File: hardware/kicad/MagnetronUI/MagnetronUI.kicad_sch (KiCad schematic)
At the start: 7 parts, among them J1 Conn_01x04, J2 Conn_02x13_Counter_Clockwise, SW1 SW_Push

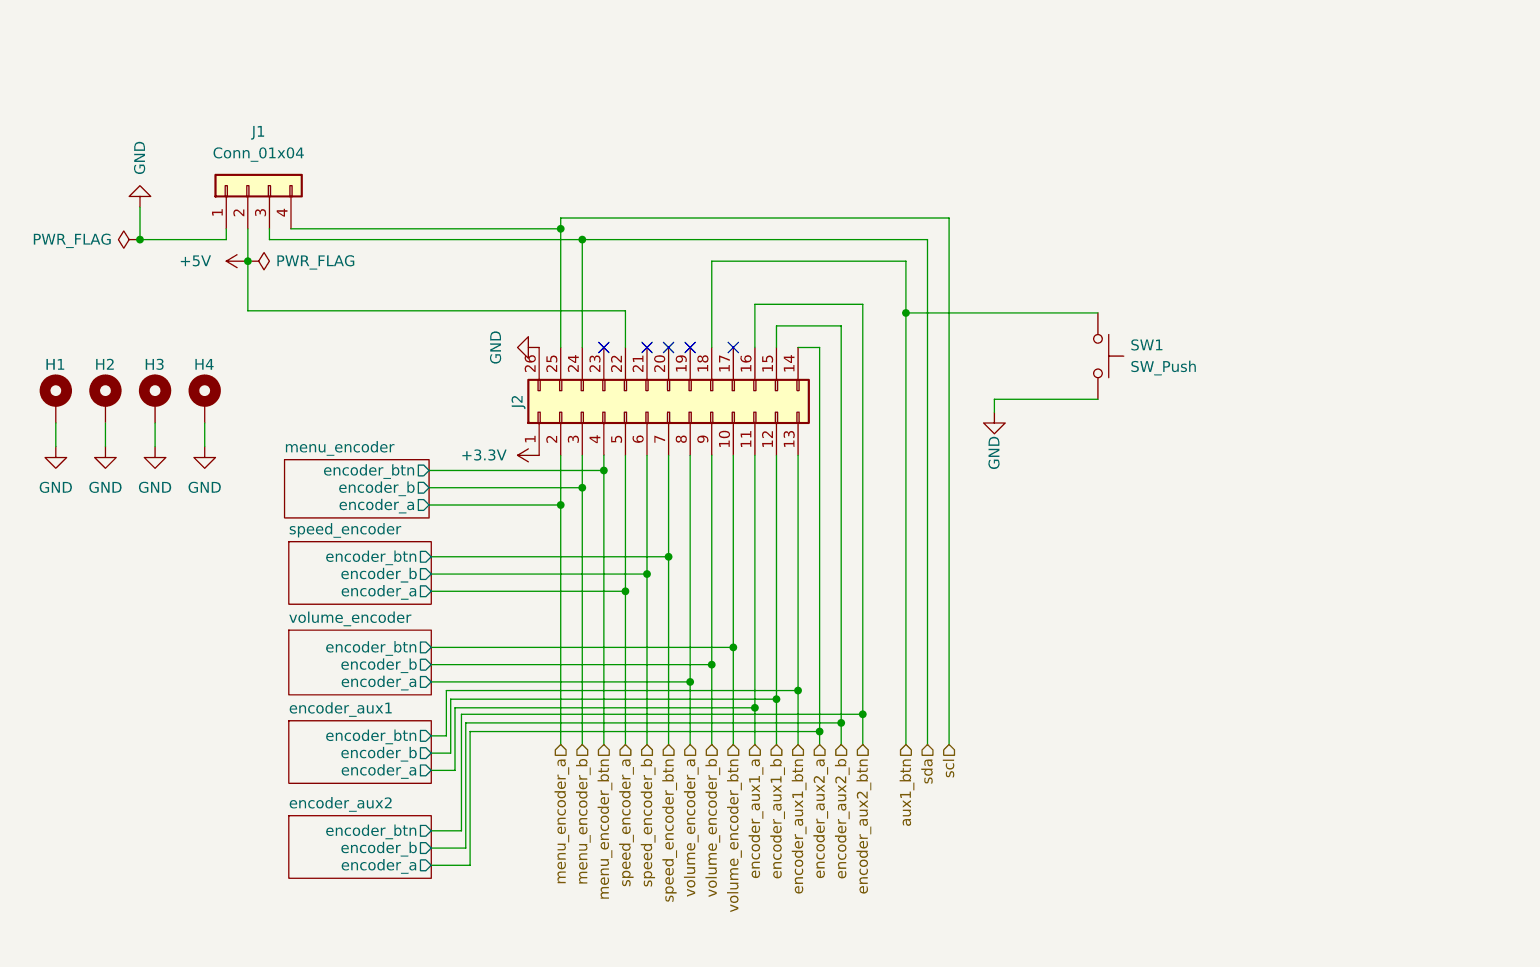
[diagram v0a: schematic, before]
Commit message: chore: cleanup
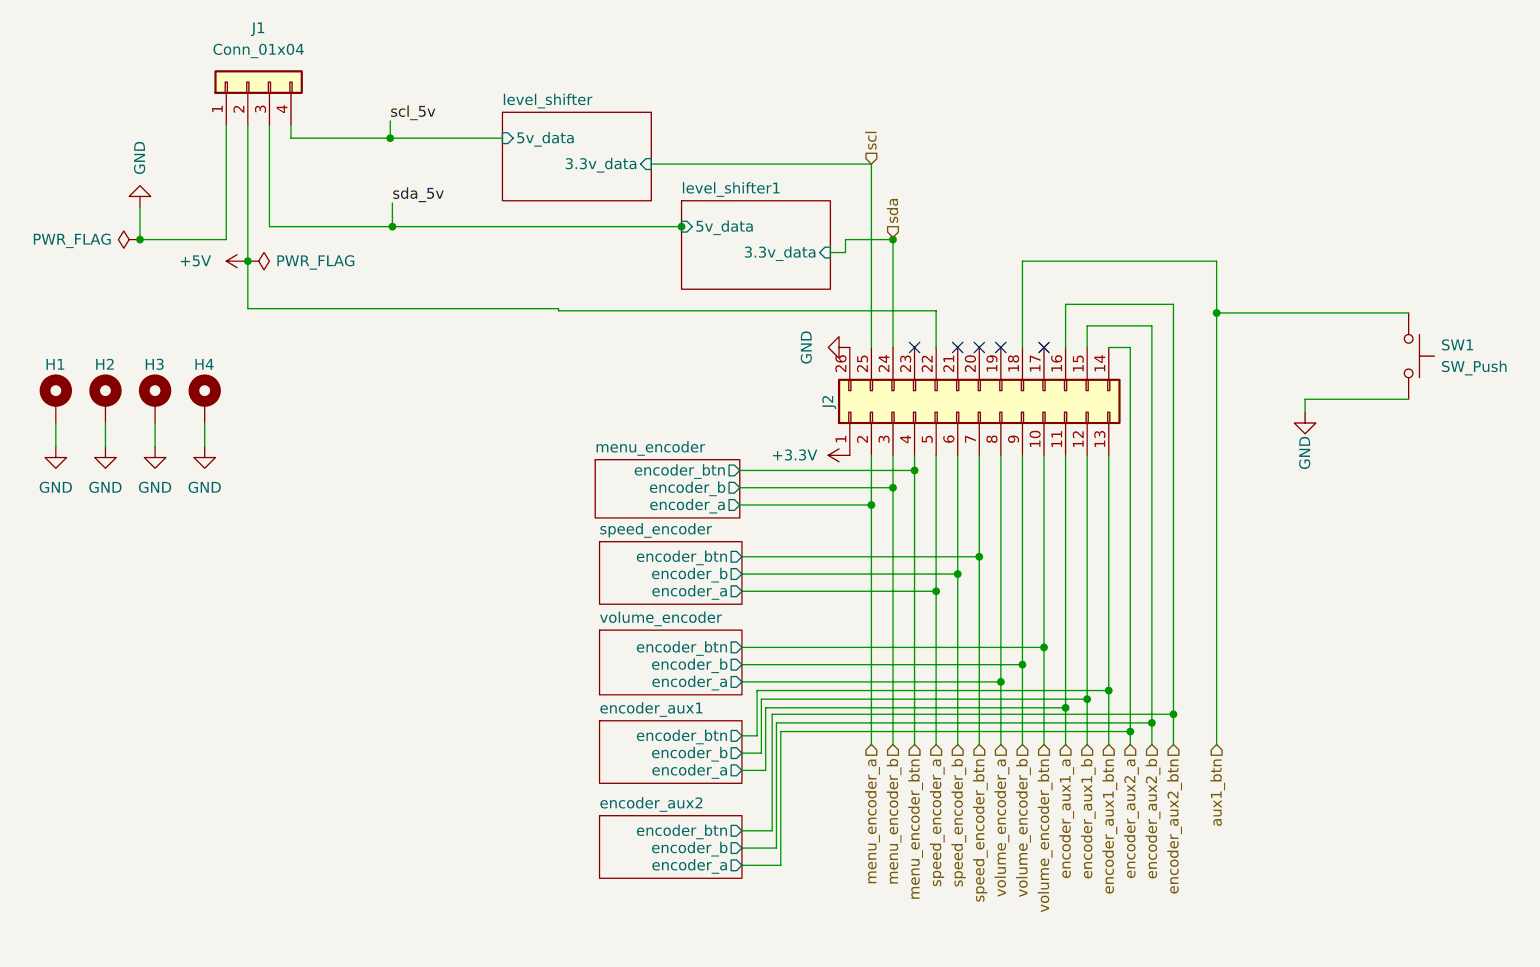
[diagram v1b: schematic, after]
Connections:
- net scl: no longer J1.4 (Pin_4)
- net sda: no longer J1.3 (Pin_3)
- new net scl_5v: J1.4 (Pin_4)
- new net sda_5v: J1.3 (Pin_3)
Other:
- added sheet level_shifter (level_shifter.kicad_sch)
- added sheet level_shifter1 (level_shifter.kicad_sch)
- moved on the sheet: J1, J2, SW1
